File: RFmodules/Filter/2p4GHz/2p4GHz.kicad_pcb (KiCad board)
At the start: 2 copper layers, 32 x 18 mm, 8 parts, among them J1 SMA, J2 SMA

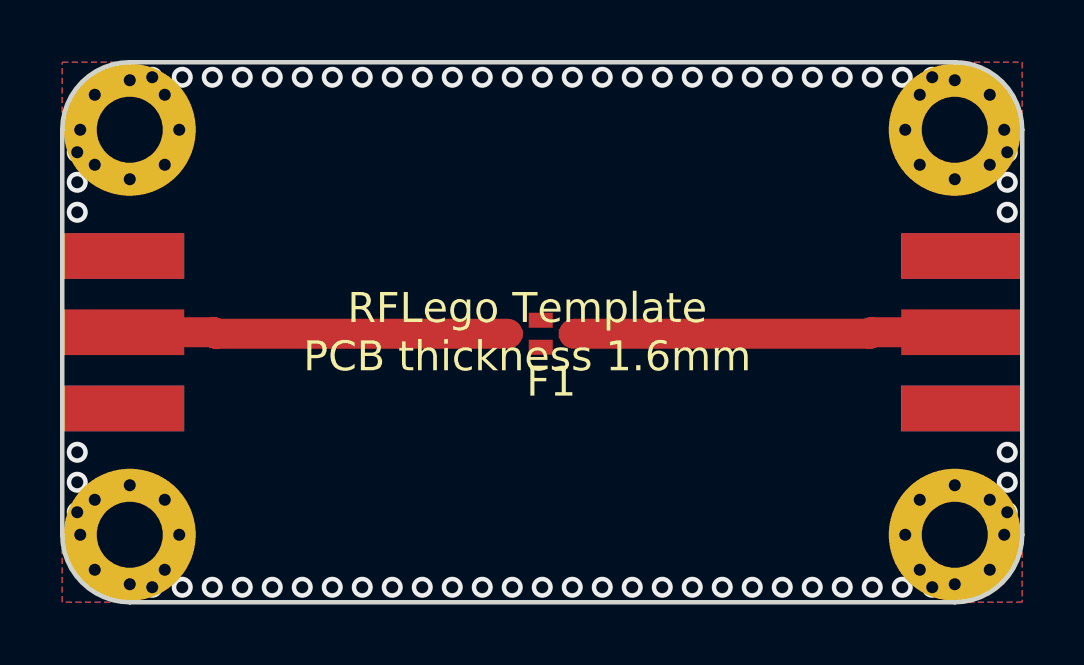
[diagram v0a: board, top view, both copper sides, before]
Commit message: Layout update
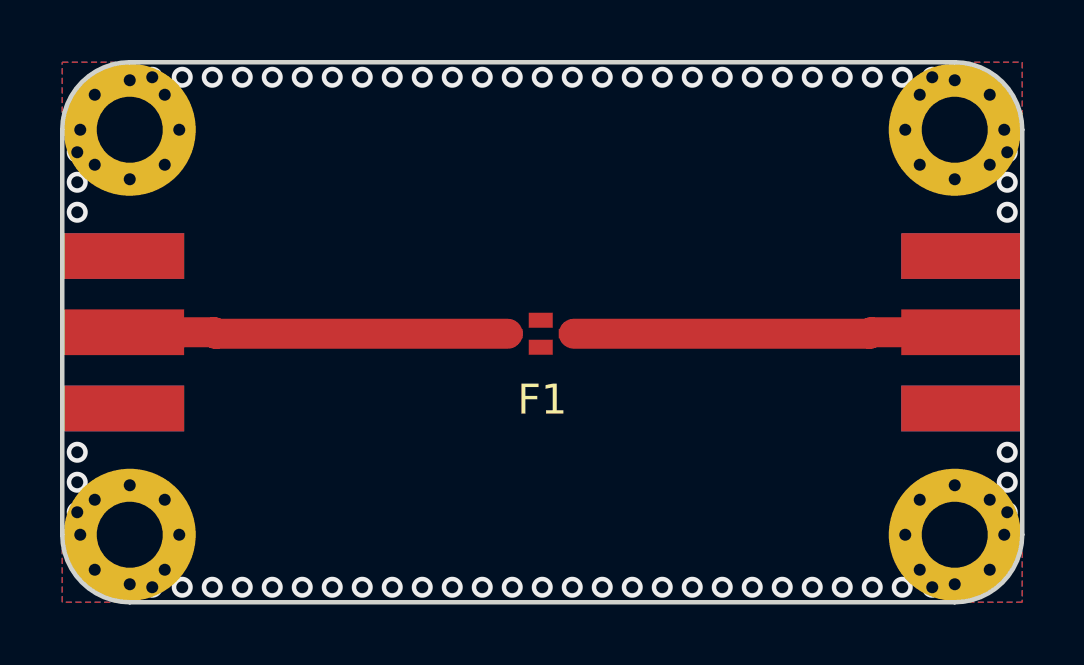
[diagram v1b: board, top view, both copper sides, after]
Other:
- board text removed: "RFLego Template PCB thickness 1.6mm"
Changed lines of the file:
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@@
   (general
     (thickness 1.6)
-    (drawings 36)
+    (drawings 35)
     (tracks 72)
     (zones 0)
@@
     (35 F.Paste user)
     (36 B.SilkS user hide)
-    (37 F.SilkS user hide)
+    (37 F.SilkS user)
     (38 B.Mask user hide)
     (39 F.Mask user hide)
@@
   (module RFLego_Footprint:DEA162450BT (layer F.Cu)
     (at 115.1 109.05)
-    (fp_text reference F1 (at 1.2 1.6) (layer F.SilkS)
+    (fp_text reference F1 (at 0.9 2.2) (layer F.SilkS)
       (effects (font (size 1 1) (thickness 0.15)))
     )
@@
       (net 3 "Net-(F1-Pad2)"))
   )
-  (gr_text "RFLego Template\nPCB thickness 1.6mm" (at 115.5 109) (layer F.SilkS)
-    (effects (font (size 1 1) (thickness 0.25)))
-  )
   (dimension 18 (width 0.3) (layer Cmts.User)
